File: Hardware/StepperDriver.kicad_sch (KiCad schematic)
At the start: 4 parts, among them M1 Stepper_Motor_bipolar, U3 L293D

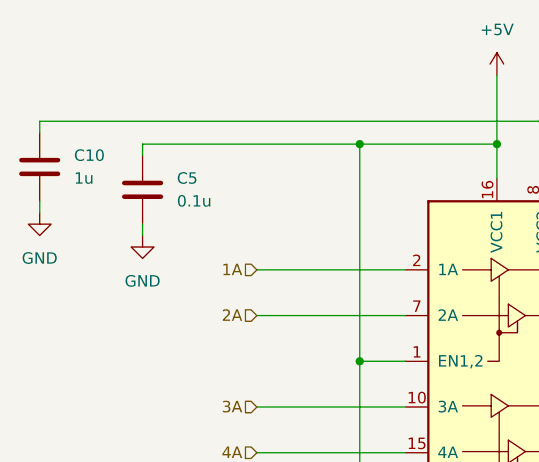
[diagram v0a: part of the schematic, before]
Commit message: PCB Updates
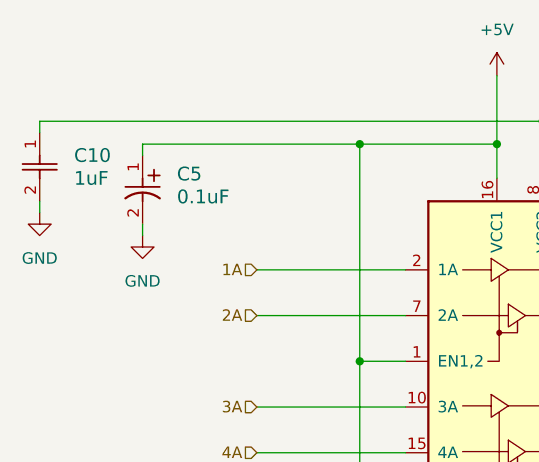
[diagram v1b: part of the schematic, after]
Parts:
- removed C10: 1u, symbol Device:C
- removed C5: 0.1u, symbol Device:C
- added C10: 1uF, ThorParts:CAP_C330C_MR_X7R_KEM, symbol 2024-10-08_03-02-35:C330C105K5R5TA7301
- added C5: 0.1uF, ThorParts:CAP_C320_KEM, symbol 2024-10-08_02-19-51:C320C104K5R5TA
- M1: footprint Connector_PinHeader_2.54mm:PinHeader_1x04_P2.54mm_Vertical -> TerminalBlock_Phoenix:TerminalBlock_Phoenix_MPT-0,5-4-2.54_1x04_P2.54mm_Horizontal
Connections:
- net +12V: now also C10.1
- net +5V: now also C5.1
- net GND: now also C10.2, C5.2
